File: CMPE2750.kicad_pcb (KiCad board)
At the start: 6 copper layers, 158.4 x 102.4 mm, 337 parts, among them J1 Conn_02x07_Odd_Even, J10 Conn_01x02, J2 Conn_02x04_Odd_Even, J3 Conn_02x16_Odd_Even, J4 Conn_01x16, J5 Conn_01x04, J6 USB4510-03-1-A, J7 Conn_02x02_Odd_Even, J8 Conn_02x02_Odd_Even, J9 Conn_01x02, Q1 IRLML6402TRPBF, Q10 2N7002, Q11 2N7002, Q12 2N7002, Q13 2N7002, Q14 2N7002, Q15 2N7002, Q16 2N7002, Q17 2N7002, Q18 2N7002, Q19 IRLML6402TRPBF, Q2 IRLML6402TRPBF, Q20 IRLML6402TRPBF, Q21 IRLML6402TRPBF, Q22 IRLML6402TRPBF, Q23 IRLML6402TRPBF, Q24 IRLML6402TRPBF, Q25 IRLML6402TRPBF, Q26 IRLML6402TRPBF, Q27 IRLML6402TRPBF, Q28 2N7002, Q29 2N7002, Q3 IRLML6402TRPBF, Q30 2N7002, Q31 2N7002, Q32 2N7002, Q33 2N7002, Q34 2N7002, Q35 2N7002, Q36 2N7002, Q37 2N7002, Q38 2N7002, Q39 2N7002, Q4 IRLML6402TRPBF, Q40 2N7002, Q41 2N7002, Q42 2N7002, Q43 2N7002, Q44 2N7002, Q45 2N7002, Q46 2N7002, Q47 2N7002, Q48 2N7002, Q49 2N7002, Q5 IRLML6402TRPBF, Q50 2N7002, Q51 2N7002, Q52 2N7002, Q53 2N7002, Q54 2N7002, Q55 2N7002, Q56 2N7002, Q57 2N7002, Q58 2N7002, Q59 2N7002, Q6 IRLML6402TRPBF, Q60 2N7002, Q61 2N7002, Q62 2N7002, Q63 2N7002, Q64 2N7002, Q65 2N7002, Q66 2N7002, Q7 IRLML6402TRPBF, Q8 IRLML6402TRPBF, Q9 IRLML6402TRPBF, SW1 D6R90F1LFS, SW2 DS04-254-1L-08BK, SW3 DS04-254-1L-08BK, U1 STM32L476RGTx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

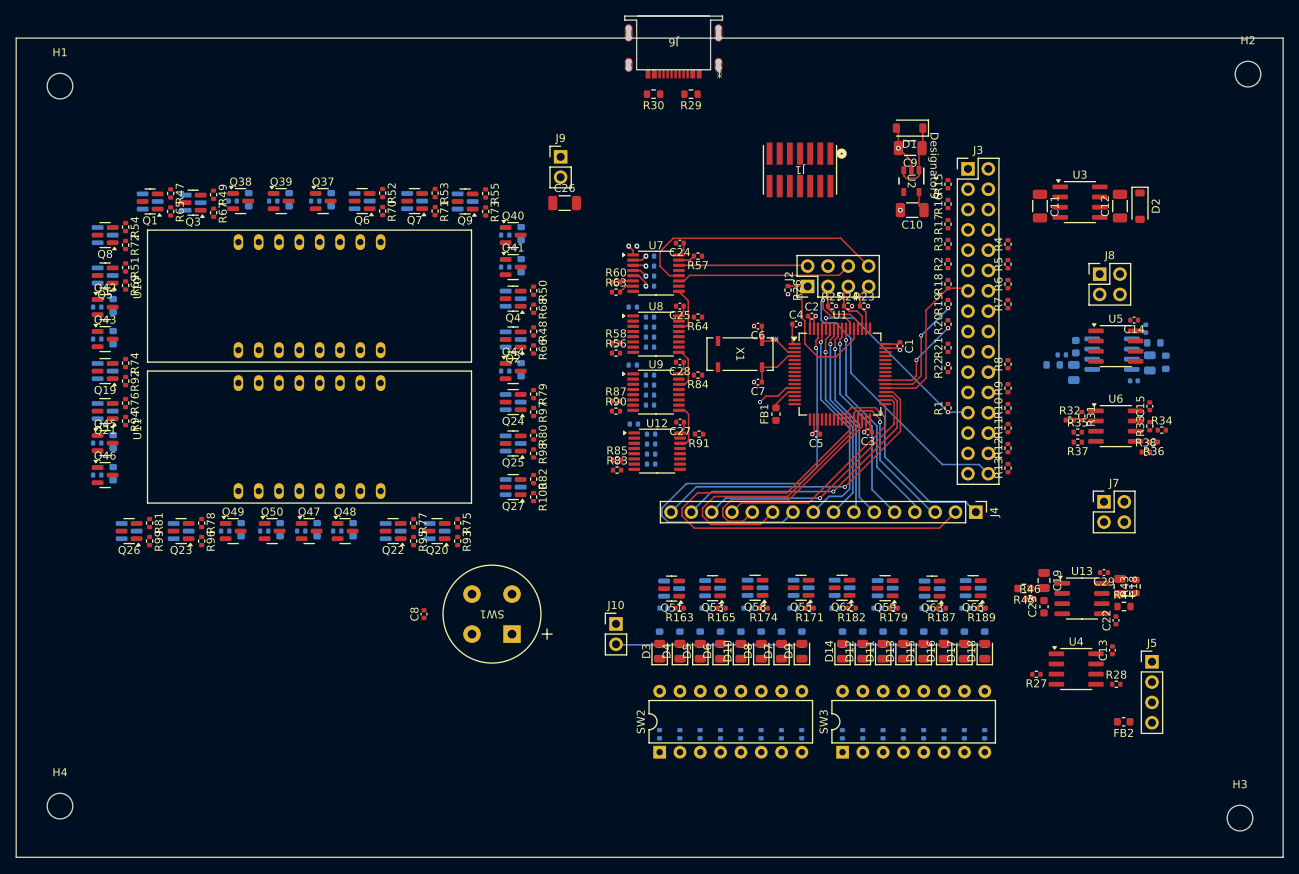
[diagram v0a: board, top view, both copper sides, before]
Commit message: pcb almost done, just need to do the final copper fill
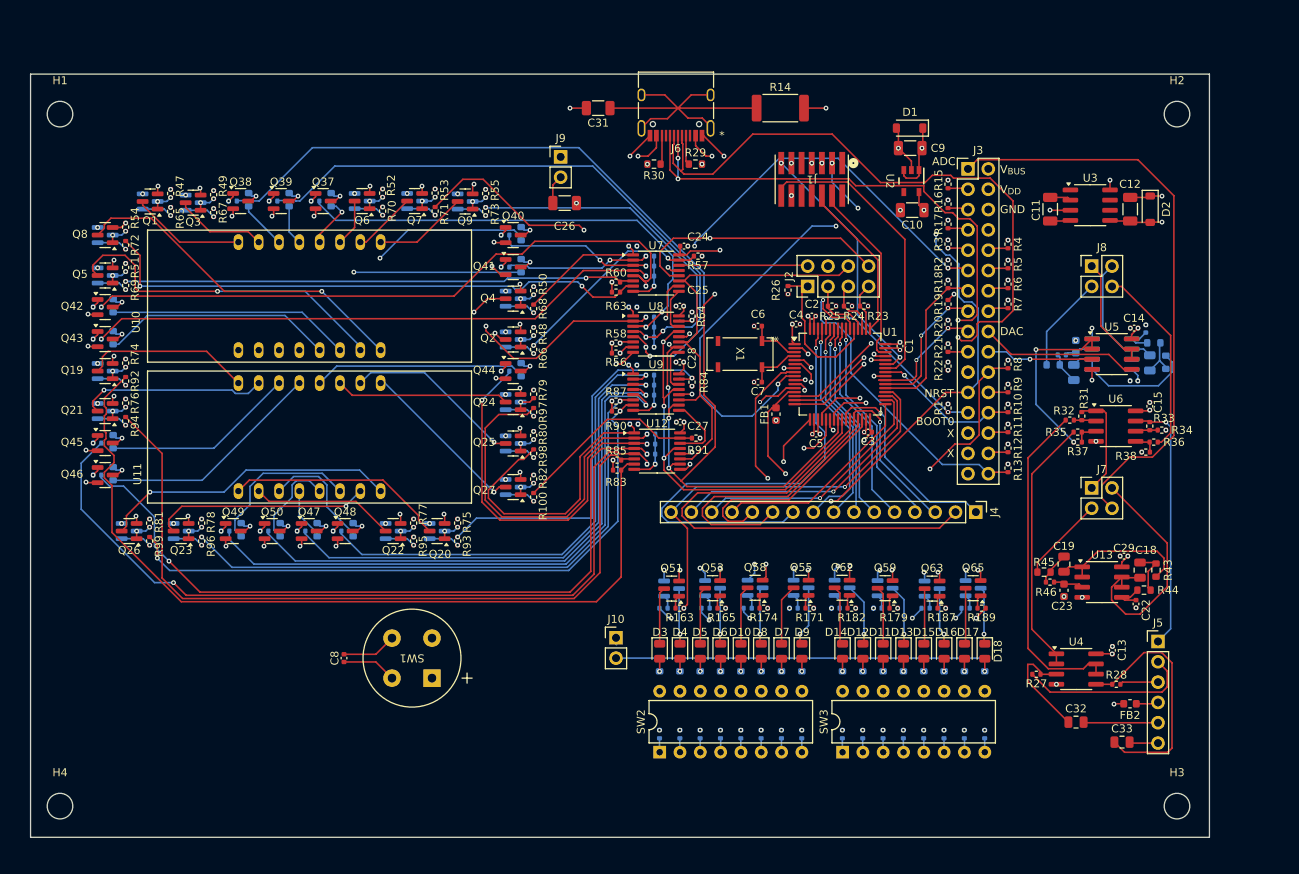
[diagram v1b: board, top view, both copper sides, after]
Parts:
- added C31: 4.7nF 1kV, Capacitor_SMD:C_1206_3216Metric, F.Cu at (124.8, 50.2)
- added C32: 1.6nF, Capacitor_SMD:C_0805_2012Metric, F.Cu at (184.5, 127.0)
- added C33: 1.6nF, Capacitor_SMD:C_0805_2012Metric, F.Cu at (190.2, 129.5)
- added R14: 1MΩ, Resistor_SMD:R_2512_6332Metric, F.Cu at (147.5, 50.2)
- C6, C7: value 3.8 pF -> 5pF
- J5: footprint Connector_PinHeader_2.54mm:PinHeader_1x04_P2.54mm_Vertical -> Connector_PinHeader_2.54mm:PinHeader_1x06_P2.54mm_Vertical
- J6: value USB4510-03-1-A -> TYPE-C-31-M-12; footprint CMPE2750:USB4510-03-1-A_GCT -> Connector_USB:USB_C_Receptacle_HRO_TYPE-C-31-M-12
- moved C8 11.4 mm to (93.0, 119.0)
- moved SW1 11.4 mm to (104.0, 121.5)
- moved H2 10.2 mm to (197.1, 51.0)
- moved R29 8.77 mm to (136.9, 57.2), turned to 0 degrees
- moved R30 8.75 mm to (131.8, 57.2)
- moved H3 8.02 mm to (197.1, 137.5)
- moved J6 7.66 mm to (134.5, 49.6)
- moved H1 3.50 mm to (57.5, 51.0)
- moved R159 3.31 mm to (132.4, 119.8), turned to 90 degrees
- moved R160 3.31 mm to (135.0, 119.8), turned to 90 degrees
- moved R161 3.31 mm to (137.5, 119.8), turned to 90 degrees
- moved R162 3.31 mm to (140.1, 119.8), turned to 90 degrees
- moved R167 3.31 mm to (147.7, 119.8), turned to 90 degrees
- moved R168 3.31 mm to (145.2, 119.8), turned to 90 degrees
- moved R169 3.31 mm to (150.2, 119.8), turned to 90 degrees
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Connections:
- R29 pad 1: GND -> Net-(J6-CC1)
- R29 pad 2: Net-(J6-CC1) -> GND
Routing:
- net GND: track 19.8 -> 241.2 mm, vias 16 -> 138
- net /NRST: track 0.00 -> 145.1 mm, vias 0 -> 4
- net /ADC: track 0.00 -> 134.6 mm, vias 0 -> 1
- net /~{SRCLR}: track 0.00 -> 116.5 mm, vias 0 -> 7
- net /~{RCL}: track 0.00 -> 112.2 mm, vias 0 -> 6
- net /Display/p32: track 0.00 -> 106.1 mm
- net /Display/p30: track 0.00 -> 100.6 mm, vias 0 -> 2
- net /Display/p31: track 0.00 -> 97.7 mm
- net /D-: track 0.00 -> 95.1 mm, vias 0 -> 2
- net /Display/p29: track 0.00 -> 92.6 mm, vias 0 -> 2
- net /Display/p14: track 0.00 -> 86.3 mm, vias 0 -> 2
- net /PC3: track 0.00 -> 84.1 mm, vias 0 -> 1
- net /Display/p24: track 0.00 -> 80.3 mm, vias 0 -> 2
- net /Display/p16: track 0.00 -> 80.0 mm, vias 0 -> 2
- net /D+: track 0.00 -> 79.6 mm, vias 0 -> 4
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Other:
- board size 158.4 x 102.4 mm -> 147.4 x 95.4 mm
- board text added: "ADC"
- board text added: "BOOT0"
- board text added: "DAC"
- board text added: "GND"
- board text added: "NRST"
- board text added: "V_{BUS}"
- board text added: "V_{DD}"
- board text added: "X"
